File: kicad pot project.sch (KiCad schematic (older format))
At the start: 9 parts

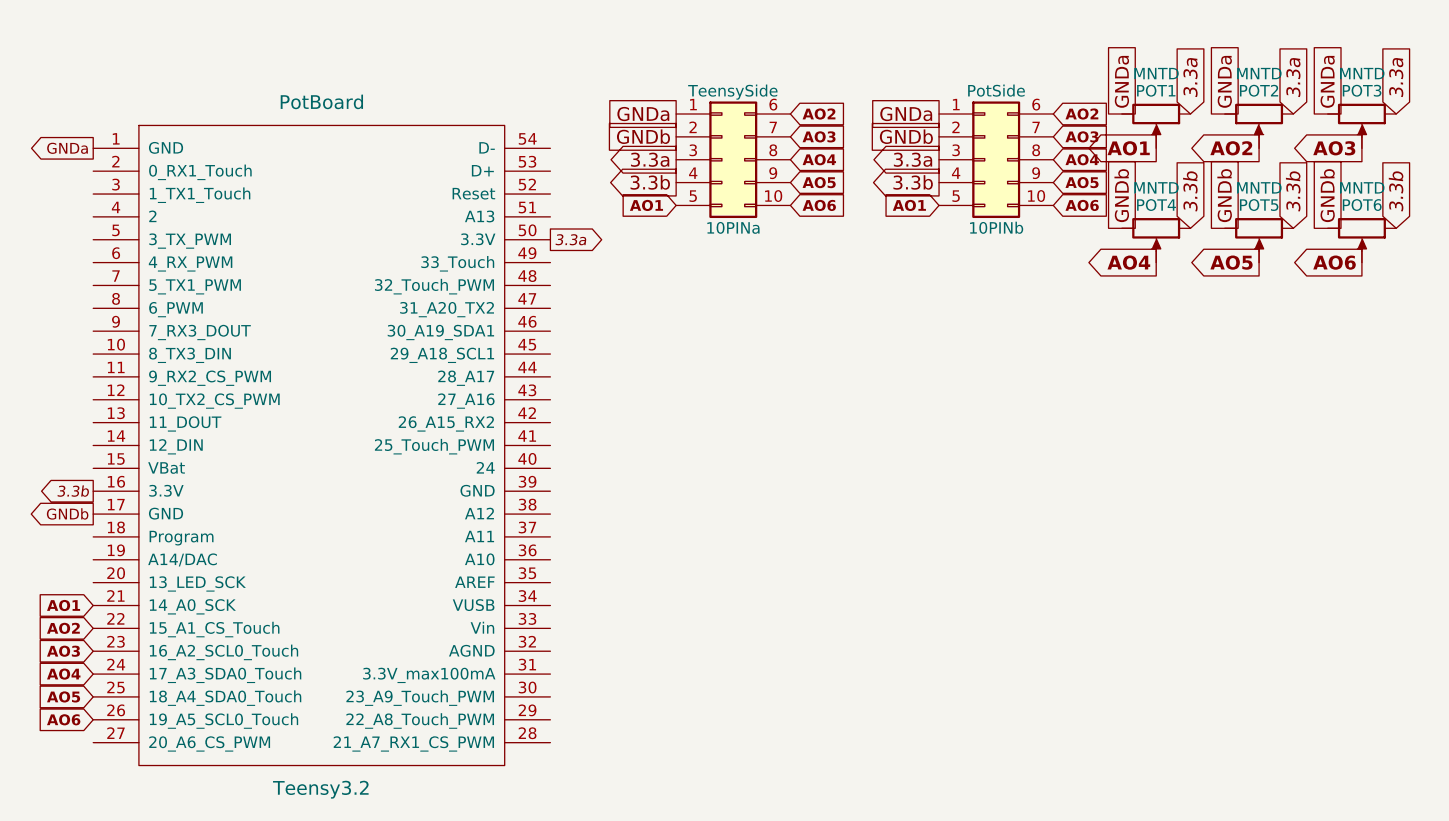
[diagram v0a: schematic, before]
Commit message: Add files via upload
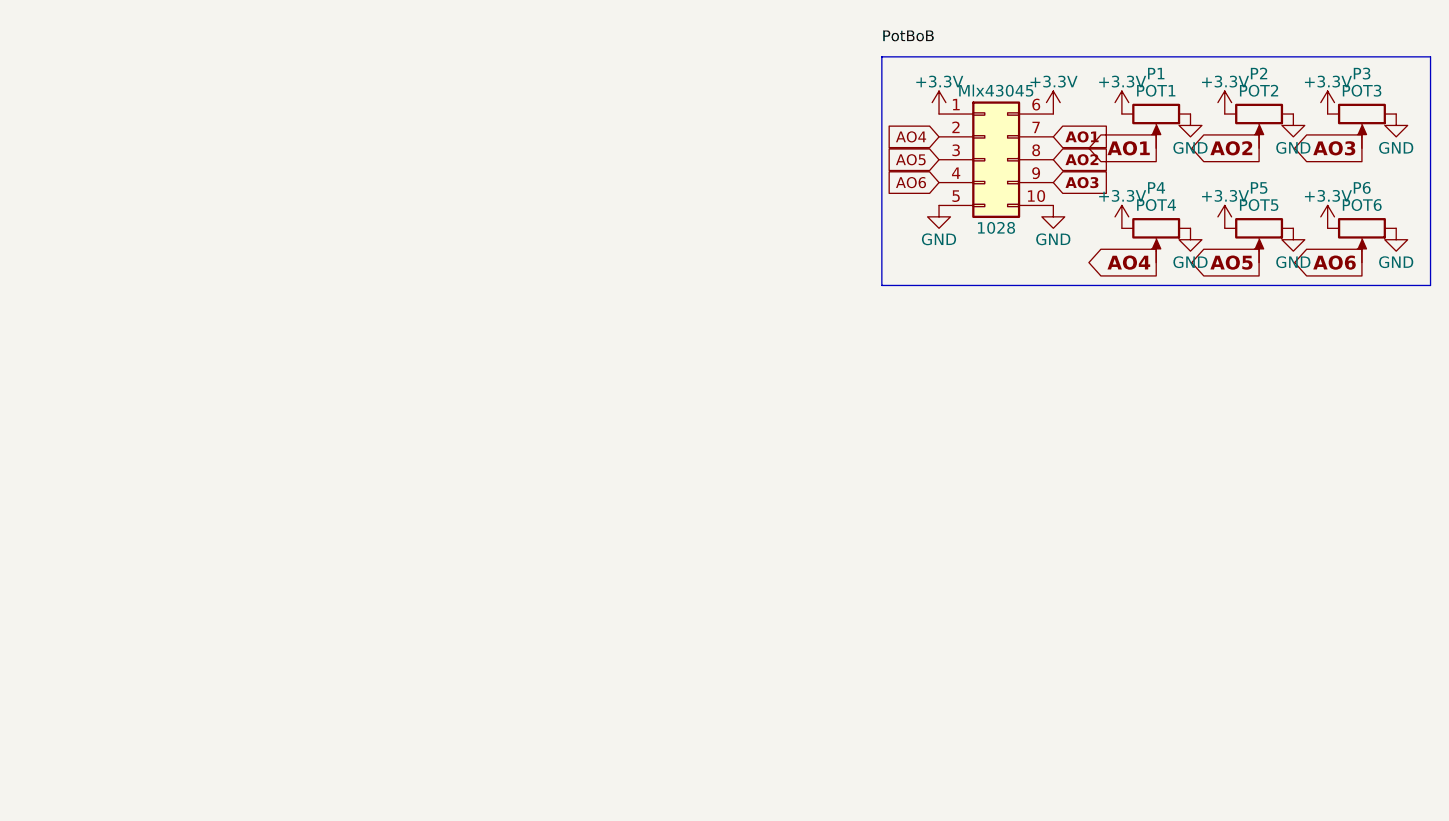
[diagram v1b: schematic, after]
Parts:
- removed MNTD: POT2, symbol POT
- removed PotBoard: Teensy3.2, symbol Teensy3.2
- removed TeensySide: 10PINa, symbol Conn_02x05_Top_Bottom
- added P2: POT2, Potentiometers:Potentiometer_Alps_RK09Y_Vertical, symbol POT
- Mlx43045: renamed from PotSide; value 10PINb -> 1028; footprint (none) -> Connectors_Molex:Molex_Microfit3_Header_02x05_Straight_43045-1028
- P1, P3, P4, P5, P6: renamed from MNTD; footprint (none) -> Potentiometers:Potentiometer_Alps_RK09Y_Vertical
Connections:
- net AO1: now also Mlx43045.7 (Pin_7); no longer Mlx43045.5 (Pin_5)
- net AO2: now also Mlx43045.8 (Pin_8), P2.2; no longer Mlx43045.6 (Pin_6)
- net AO3: now also Mlx43045.9 (Pin_9); no longer Mlx43045.7 (Pin_7)
- net AO4: now also Mlx43045.2 (Pin_2); no longer Mlx43045.8 (Pin_8)
- net AO5: now also Mlx43045.3 (Pin_3); no longer Mlx43045.9 (Pin_9)
- net AO6: now also Mlx43045.4 (Pin_4); no longer Mlx43045.10 (Pin_10)
- net 3.3a renamed GND
- net GND: now also Mlx43045.10 (Pin_10), Mlx43045.5 (Pin_5), P4.1, P5.1, P6.1, P2.1; no longer Mlx43045.3 (Pin_3)
- removed net 3.3b: Mlx43045.4 (Pin_4), P4.1, P5.1, P6.1
- net GNDa renamed +3V3
- net +3V3: now also Mlx43045.6 (Pin_6), P4.3, P5.3, P6.3, P2.3
- removed net GNDb: Mlx43045.2 (Pin_2), P4.3, P5.3, P6.3

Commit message: Add files via upload
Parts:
- P1, P2, P3, P4, P5, P6: footprint Potentiometers:Potentiometer_Alps_RK09Y_Vertical -> Potentiometers:Potentiometer_Alps_RK09K_Horizontal
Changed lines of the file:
@@
 F 0 "P3" V 9775 1150 50  0000 C CNN
 F 1 "POT3" V 9850 1150 50  0000 C CNN
-F 2 "Potentiometers:Potentiometer_Alps_RK09Y_Vertical" H 9950 1150 50  0001 C CNN
+F 2 "Potentiometers:Potentiometer_Alps_RK09K_Horizontal" H 9950 1150 50  0001 C CNN
 F 3 "" H 9950 1150 50  0001 C CNN
 	1    9950 1150
@@
 F 0 "P4" V 8875 1650 50  0000 C CNN
 F 1 "POT4" V 8950 1650 50  0000 C CNN
-F 2 "Potentiometers:Potentiometer_Alps_RK09Y_Vertical" H 9050 1650 50  0001 C CNN
+F 2 "Potentiometers:Potentiometer_Alps_RK09K_Horizontal" H 9050 1650 50  0001 C CNN
 F 3 "" H 9050 1650 50  0001 C CNN
 	1    9050 1650
@@
 F 0 "P5" V 9325 1650 50  0000 C CNN
 F 1 "POT5" V 9400 1650 50  0000 C CNN
-F 2 "Potentiometers:Potentiometer_Alps_RK09Y_Vertical" H 9500 1650 50  0001 C CNN
+F 2 "Potentiometers:Potentiometer_Alps_RK09K_Horizontal" H 9500 1650 50  0001 C CNN
 F 3 "" H 9500 1650 50  0001 C CNN
 	1    9500 1650
@@
 F 0 "P6" V 9775 1650 50  0000 C CNN
 F 1 "POT6" V 9850 1650 50  0000 C CNN
-F 2 "Potentiometers:Potentiometer_Alps_RK09Y_Vertical" H 9950 1650 50  0001 C CNN
+F 2 "Potentiometers:Potentiometer_Alps_RK09K_Horizontal" H 9950 1650 50  0001 C CNN
 F 3 "" H 9950 1650 50  0001 C CNN
 	1    9950 1650
@@
 F 0 "P1" V 8875 1150 50  0000 C CNN
 F 1 "POT1" V 8950 1150 50  0000 C CNN
-F 2 "Potentiometers:Potentiometer_Alps_RK09Y_Vertical" H 9050 1150 50  0001 C CNN
+F 2 "Potentiometers:Potentiometer_Alps_RK09K_Horizontal" H 9050 1150 50  0001 C CNN
 F 3 "" H 9050 1150 50  0001 C CNN
 	1    9050 1150
@@
 F 0 "P2" V 9325 1150 50  0000 C CNN
 F 1 "POT2" V 9400 1150 50  0000 C CNN
-F 2 "Potentiometers:Potentiometer_Alps_RK09Y_Vertical" H 9500 1150 50  0001 C CNN
+F 2 "Potentiometers:Potentiometer_Alps_RK09K_Horizontal" H 9500 1150 50  0001 C CNN
 F 3 "" H 9500 1150 50  0001 C CNN
 	1    9500 1150
